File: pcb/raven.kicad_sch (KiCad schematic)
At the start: 49 parts, among them J1 Conn_02x20_Odd_Even, J11 Conn_01x02_Pin, J2 Conn_01x04_MountingPin, J3 Conn_01x02_Pin, J4 Conn_01x02_Pin, J5 Conn_01x04_MountingPin, J6 Conn_01x02_Pin, J7 Conn_01x02_Pin, J8 Conn_01x02_Pin, J9 Conn_01x02_Pin, Q1 DMP2002UPS, U9 TPS548B28RWWR

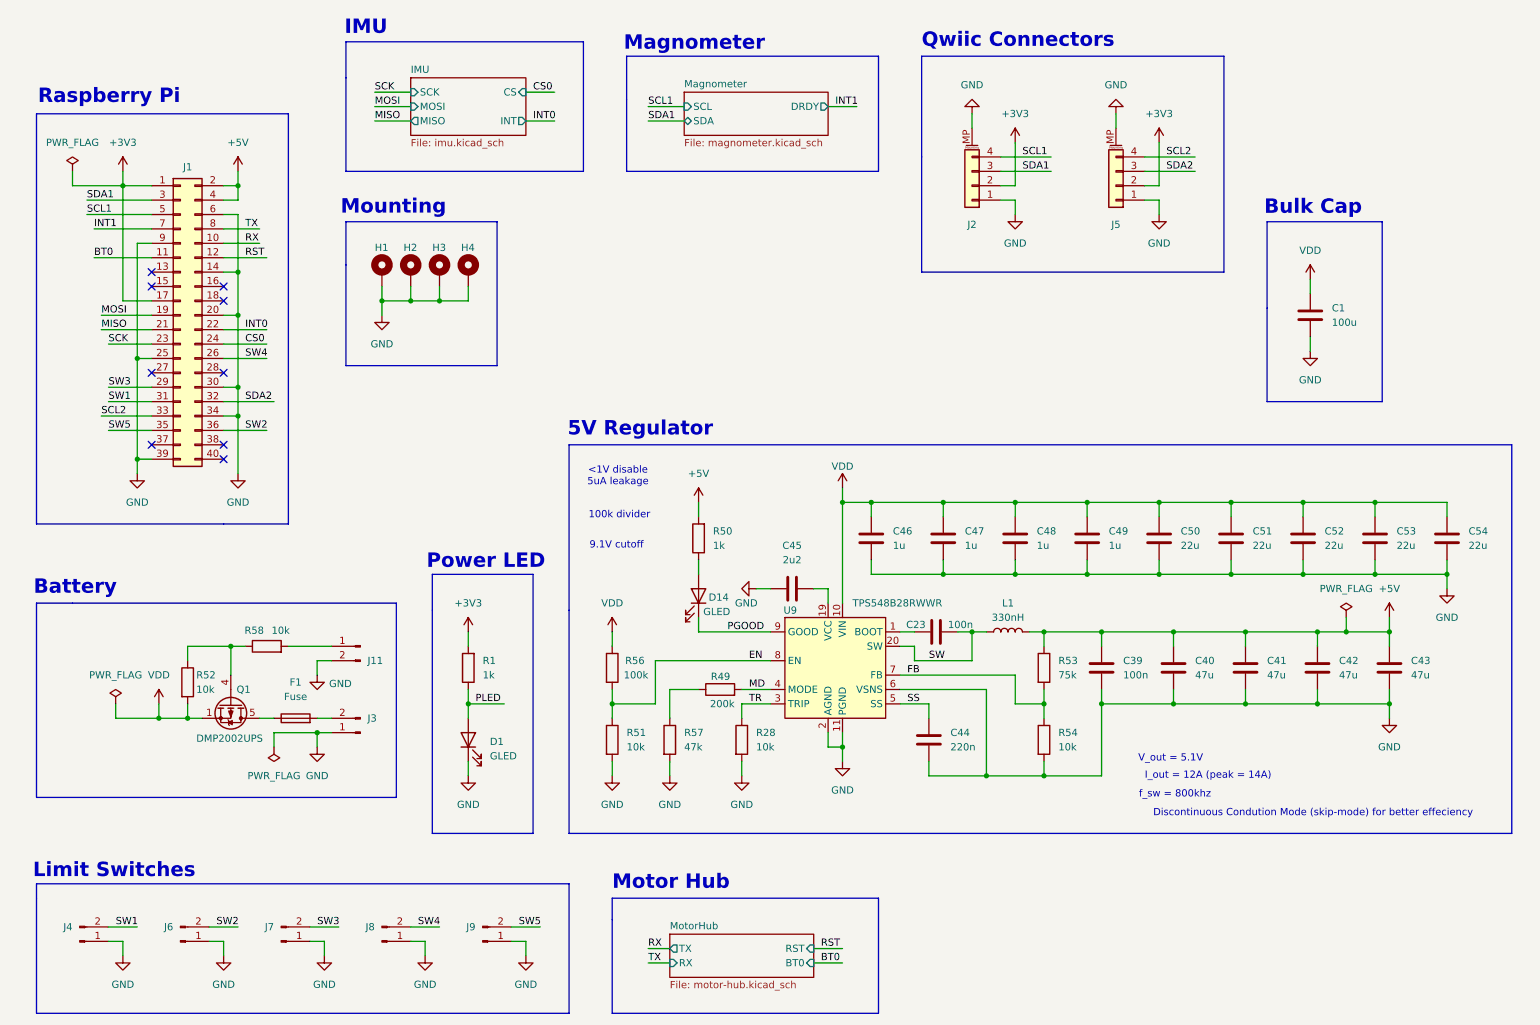
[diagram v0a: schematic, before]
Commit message: Finish for revision 2 production
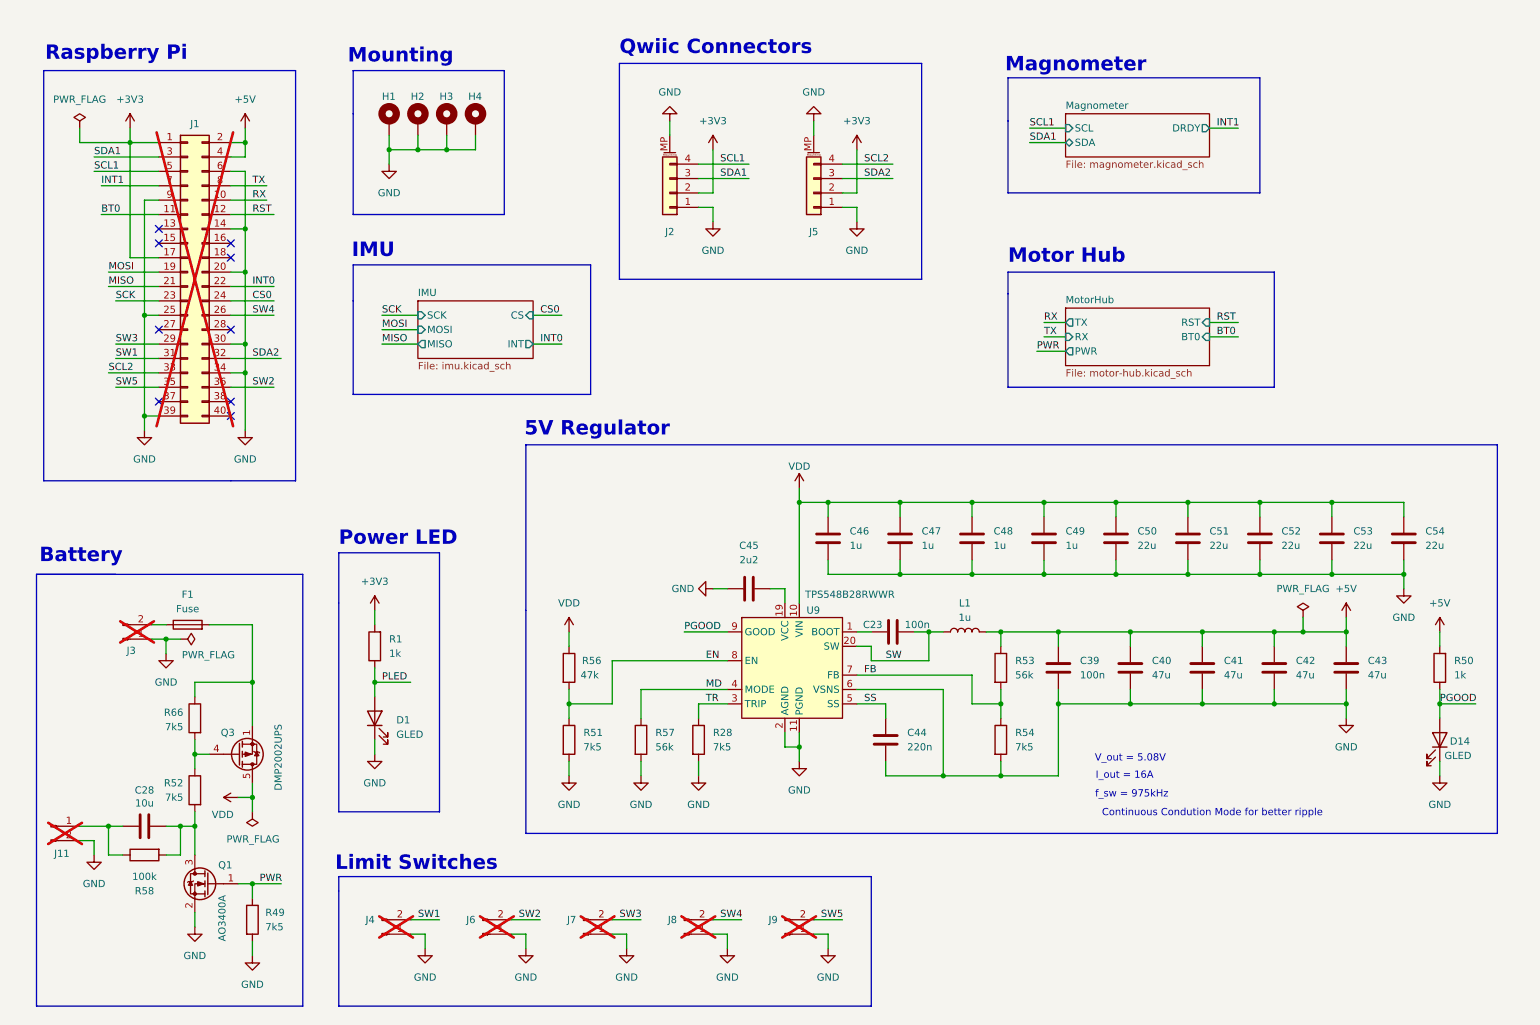
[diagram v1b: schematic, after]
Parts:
- removed C1: 100u, Capacitor_SMD:C_Elec_8x6.2, symbol Device:C
- removed Q1: DMP2002UPS, Footprints:DMP2002UPS, symbol Symbols:DMP2002UPS
- added C28: 10u, Capacitor_SMD:C_0603_1608Metric, symbol Device:C
- added Q1: AO3400A, Package_TO_SOT_SMD:SOT-23, symbol Transistor_FET:AO3400A
- added Q3: DMP2002UPS, Footprints:DMP2002UPS, symbol Symbols:DMP2002UPS
- added R66: 7k5, Resistor_SMD:R_0402_1005Metric, symbol Device:R
- J1, J11, J3, J4, J6, J7, J8, J9: now not fitted
- L1: value 330nH -> 1u; footprint Inductor_SMD:L_Changjiang_FXL0630 -> Footprints:L_0660A; LCSC C167211 -> C18199443
- R28, R51, R52, R54: value 10k -> 7k5; LCSC C25744 -> C25918
- R49: value 200k -> 7k5; LCSC C25764 -> C25918
- R53: value 75k -> 56k; LCSC C25798 -> C25796
- R56: value 100k -> 47k; LCSC C25741 -> C25792
- R57: value 47k -> 56k; LCSC C25792 -> C25796
- R58: value 10k -> 100k; LCSC C25744 -> C25741
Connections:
- net GND: now also D14.1 (K), R49.2, Q1.2 (S)
- net MD: now also R57.1; no longer R49.2
- net PGOOD: now also D14.2 (A), R50.1; no longer D14.1 (K)
- net VDD: now also Q3.5 (D), Q3.6 (D), Q3.7 (D), Q3.8 (D); no longer R52.2
- net at R58.1: now also J11.1 (Pin_1), C28.1; no longer R52.1
- net at F1.1: now also J3.2 (Pin_2)
- net at F1.2: now also Q3.1 (S), Q3.2 (S), Q3.3 (S), R66.1; no longer J3.2 (Pin_2)
- net at R58.2: now also R52.2, C28.2, Q1.3 (D); no longer J11.1 (Pin_1)
- net PWR: now reaches R49.1
- net PWR: now also Q1.1 (G); no longer R57.1
- new net: Q3.4 (G), R52.1, R66.2
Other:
- sheet MotorHub ports: added PWR; removed none
- note added: "Continuous Condution Mode for better ripple"
- note added: "I_out = 16A"
- note added: "V_out = 5.08V"
- note added: "f_sw = 975kHz"
- note removed: "100k divider"
- note removed: "9.1V cutoff"
- note removed: "<1V disable 5uA leakage"
- note removed: "Bulk Cap"
- note removed: "Discontinuous Condution Mode (skip-mode) for better effeciency"
- note removed: "I_out = 12A (peak = 14A)"
- note removed: "V_out = 5.1V"
- note removed: "f_sw = 800khz"
- moved on the sheet: C23, C39, C40, C41, C42, C43, C44, C45, C46, C47, C48, C49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
